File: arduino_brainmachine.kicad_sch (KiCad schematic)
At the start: 85 parts, among them Q1 2N5551, Q2 2N5551, Q4 2N5551, Q5 PNP, Q6 PNP, SW1 SW_Push, U1 VOS618A, U2 VOS618A, U3 LM358_DFN, U4 LM7805_TO220

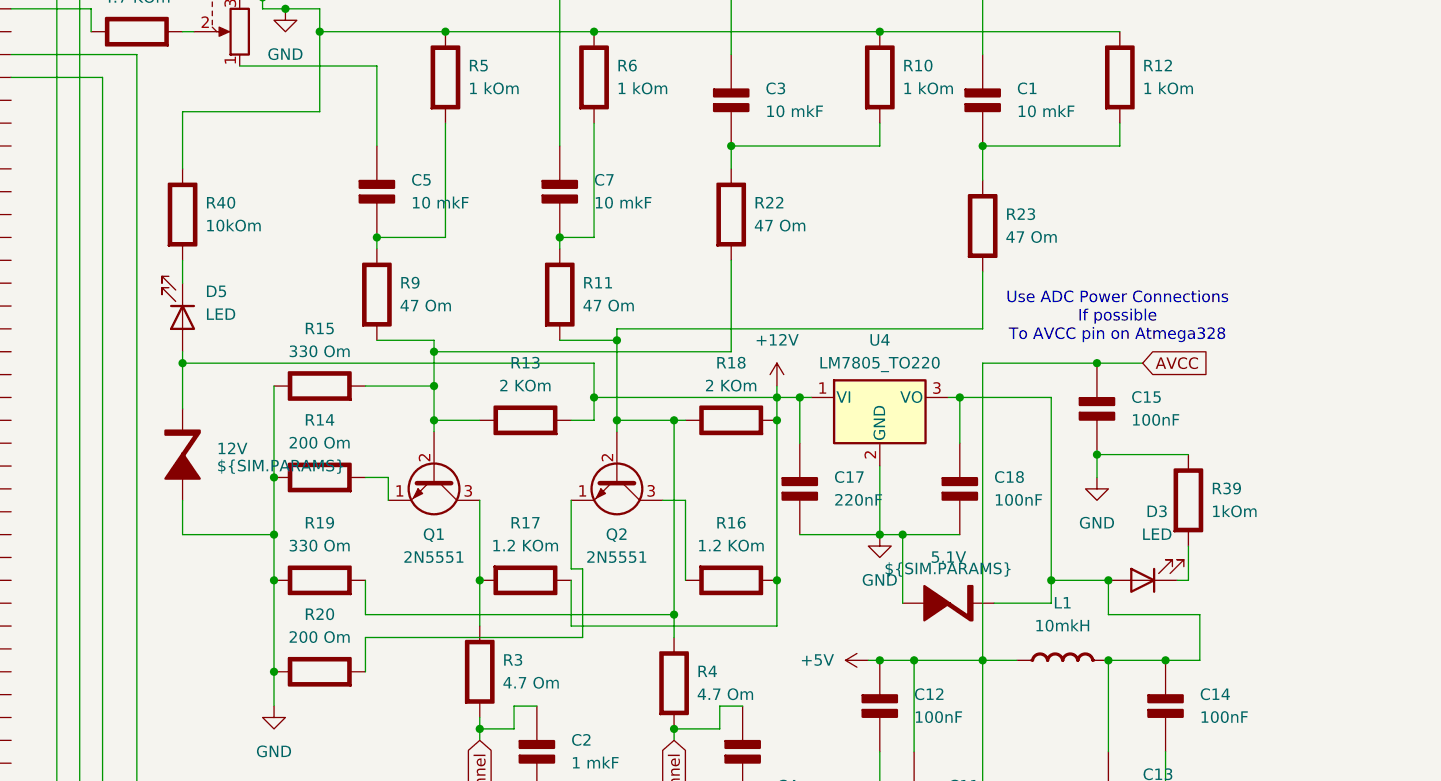
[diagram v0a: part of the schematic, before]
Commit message: Upgrade schematics | fixed
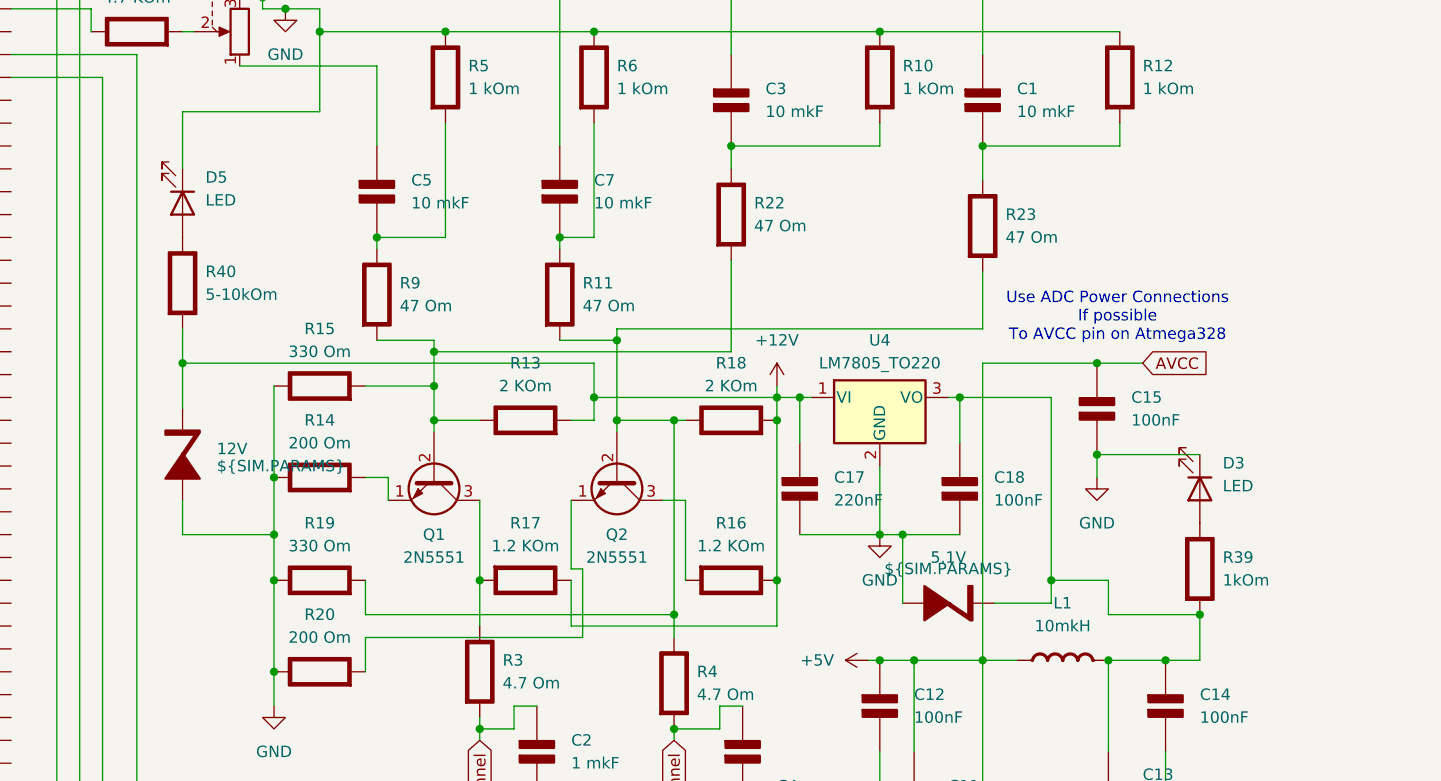
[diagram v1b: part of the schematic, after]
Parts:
- R40: value 10kOm -> 5-10kOm
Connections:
- net +12V: now also R40.2 (-); no longer D5.2 (A)
- net GND: now also D3.1 (K), D5.1 (K); no longer R39.1 (+), R40.1 (+)
- net at 5.1V.1 (K-), C13.1 (+), C14.1 (+)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: now also R39.2 (-); no longer D3.2 (A)
- new net: D5.2 (A), R40.1 (+)
- new net: D3.2 (A), R39.1 (+)
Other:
- moved on the sheet: D5, R39
